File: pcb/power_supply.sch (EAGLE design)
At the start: 45 parts, among them IC1 AP1507-D5-13, P1 2k, Q1 DIODES_FMMT493ATADIODES_FMMT4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, Q2 DIODES_FMMT493ATADIODES_FMMT4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, Q3 DIODES_FMMT493ATADIODES_FMMT4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, Q4 DIODES_FMMT493ATADIODES_FMMT4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, Q5 DIODES_FMMT493ATADIODES_FMMT4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, Q6 DIODES_FMMT493ATADIODES_FMMT4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, Q7 DIODES_FMMT493ATADIODES_FMMT4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, Q8 DIODES_FMMT493ATADIODES_FMMT4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, U1 LM1085IT-ADJ

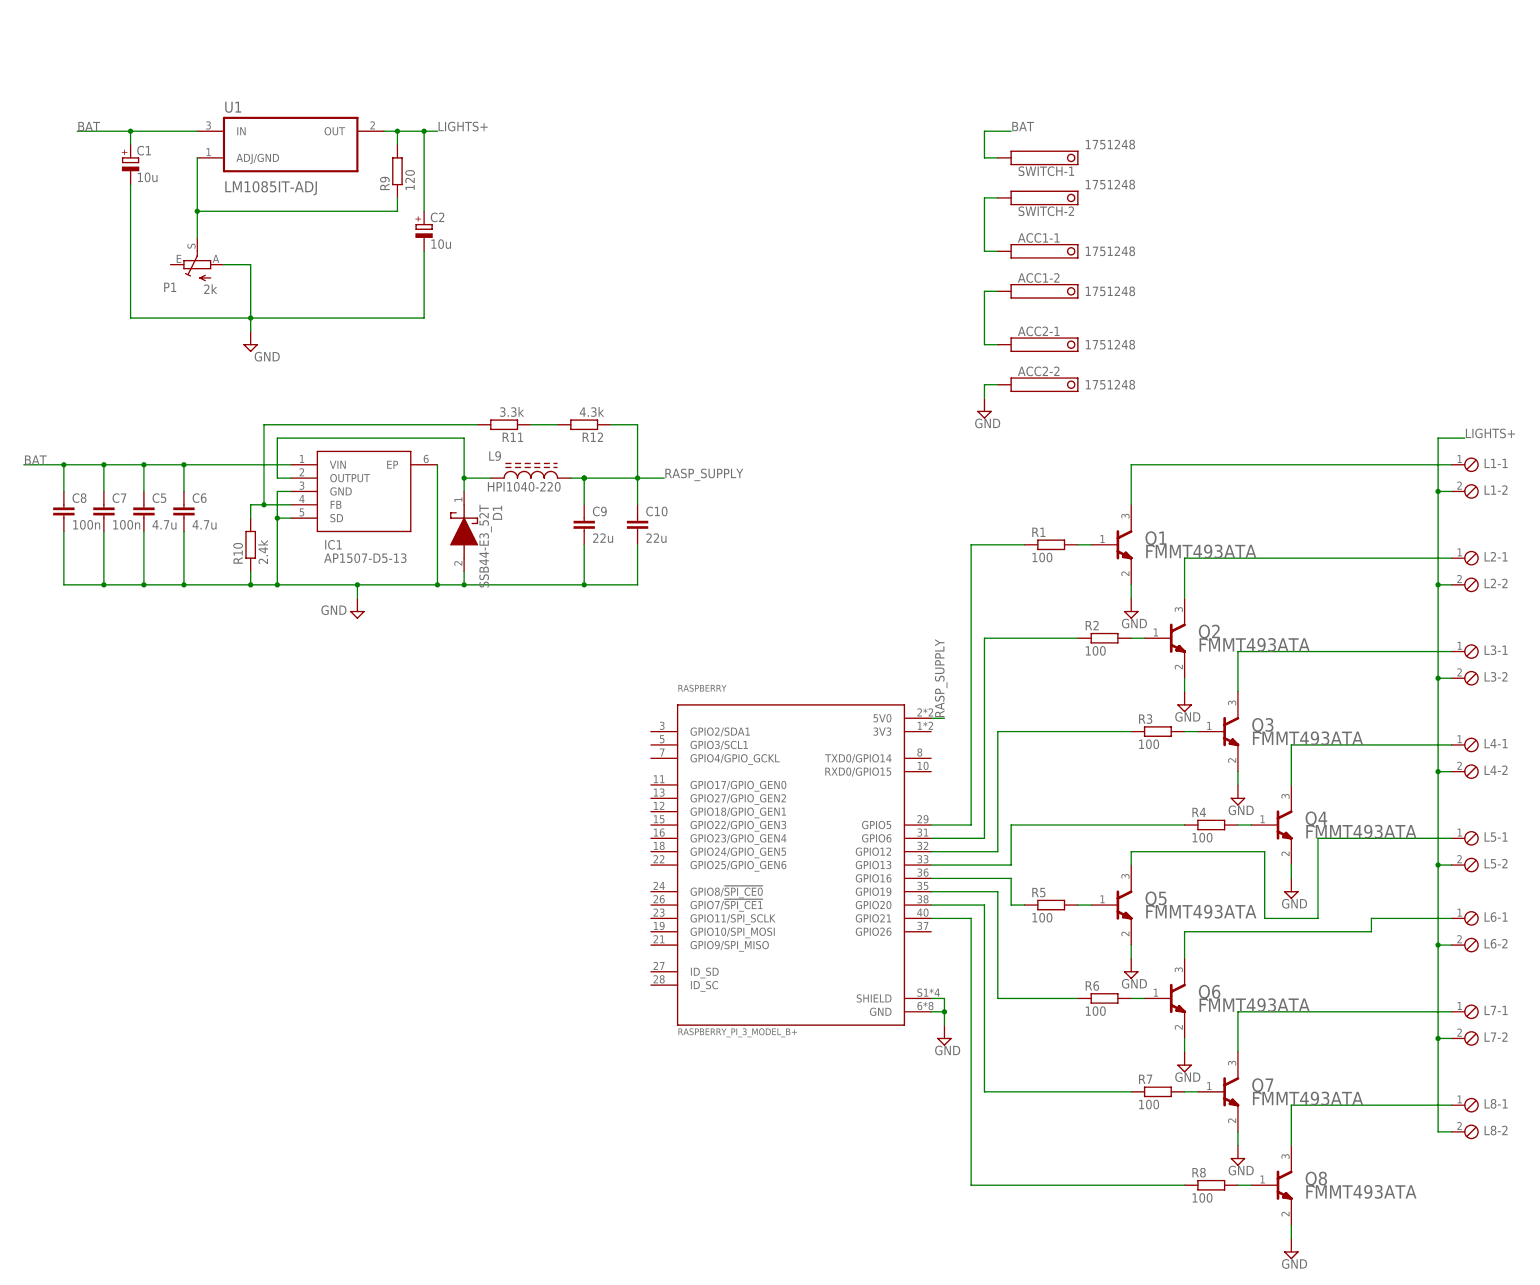
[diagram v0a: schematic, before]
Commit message: pcb - schemat updated
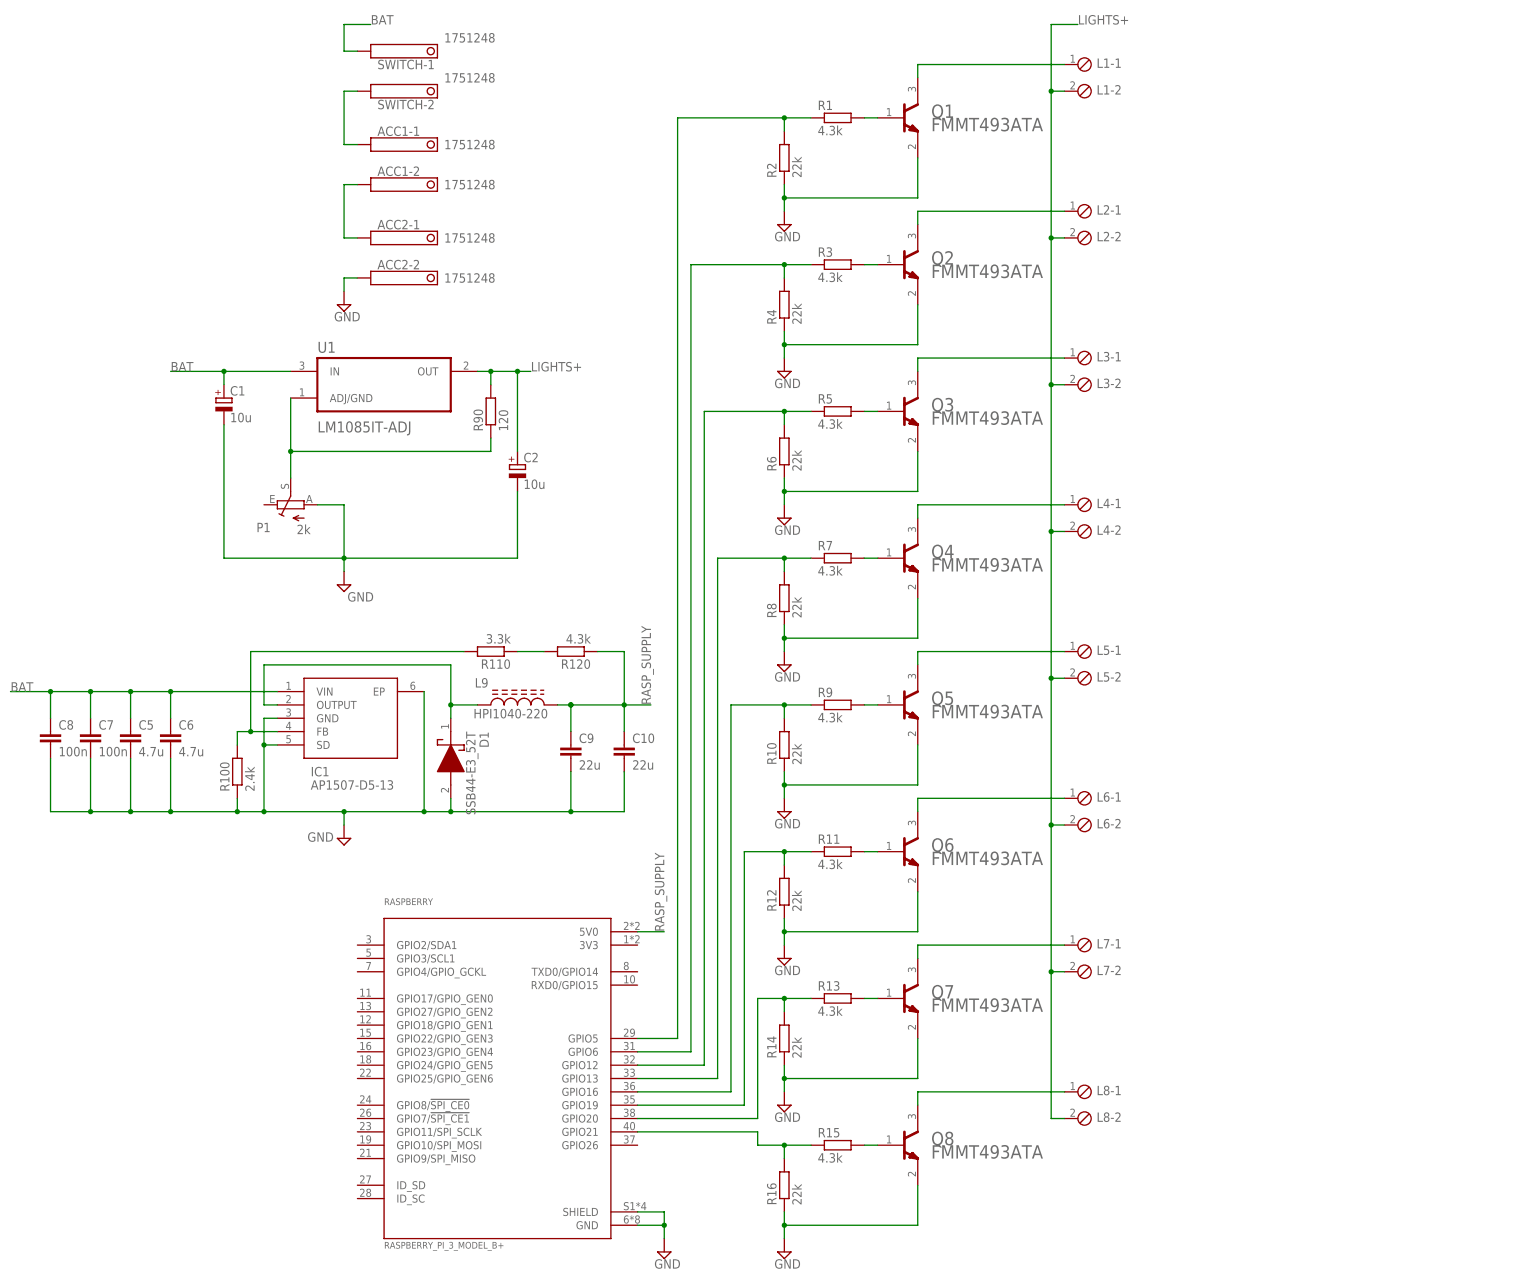
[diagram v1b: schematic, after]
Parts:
- added R100: 2.4k, rcl:R-EU_R0805
- added R110: 3.3k, rcl:R-EU_R0805
- added R120, R13, R15: 4.3k, rcl:R-EU_R0805
- added R14, R16: 22k, rcl:R-EU_R0805
- added R90: 120, rcl:R-EU_R0805
- L2, L3, L4, L5, L6, L7, L8: value (none) -> 1
- R1, R3, R5, R7: value 100 -> 4.3k
- R10: value 2.4k -> 22k
- R11: value 3.3k -> 4.3k
- R12: value 4.3k -> 22k
- R2, R4, R6, R8: value 100 -> 22k
- R9: value 120 -> 4.3k
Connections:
- removed net N$11: Q5.B, R5.2
- removed net N$15: Q7.B, R7.2
- removed net N$7: Q3.B, R3.2
- new net N$33: Q6.B, R11.2
- new net N$37: Q7.B, R13.2
- new net N$41: Q8.B, R15.2
- net GND: now also R100.1, R12.1, R14.1, R16.1, R2.1, R4.1, R6.1, R8.1
- net LIGHTS+: now also R90.2; no longer R9.2
- net N$13: now also Q4.B, R7.2; no longer Q6.B, R6.2
- net N$17: now also Q5.B, R9.2; no longer Q8.B, R8.2
- net N$19: now also R2.2
- net N$20: now also R3.1, R4.2; no longer R2.1
- net N$21: now also R5.1, R6.2; no longer R3.1
- net N$23: now also R7.1, R8.2; no longer R4.1
- net N$24: now also R10.2, R9.1; no longer R5.1
- net N$25: now also R11.1, R12.2; no longer R6.1
- net N$26: now also R13.1, R14.2; no longer R7.1
- net N$27: now also R15.1, R16.2; no longer R8.1
- net N$28: now also R110.1, R120.2; no longer R11.1, R12.2
- net N$29: now also R90.1; no longer R9.1
- net N$5: now also R3.2; no longer R2.2
- net N$9: now also Q3.B, R5.2; no longer Q4.B, R4.2
- net RASP_SUPPLY: now also R100.2, R110.2, R120.1; no longer R10.2, R11.2, R12.1
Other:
- moved on the sheet: ACC1-1, ACC1-2, ACC2-1, ACC2-2, C1, C10, C2, C5, C6, C7, C8, C9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
